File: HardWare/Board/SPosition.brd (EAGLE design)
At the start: 60 x 110 mm, 72 parts

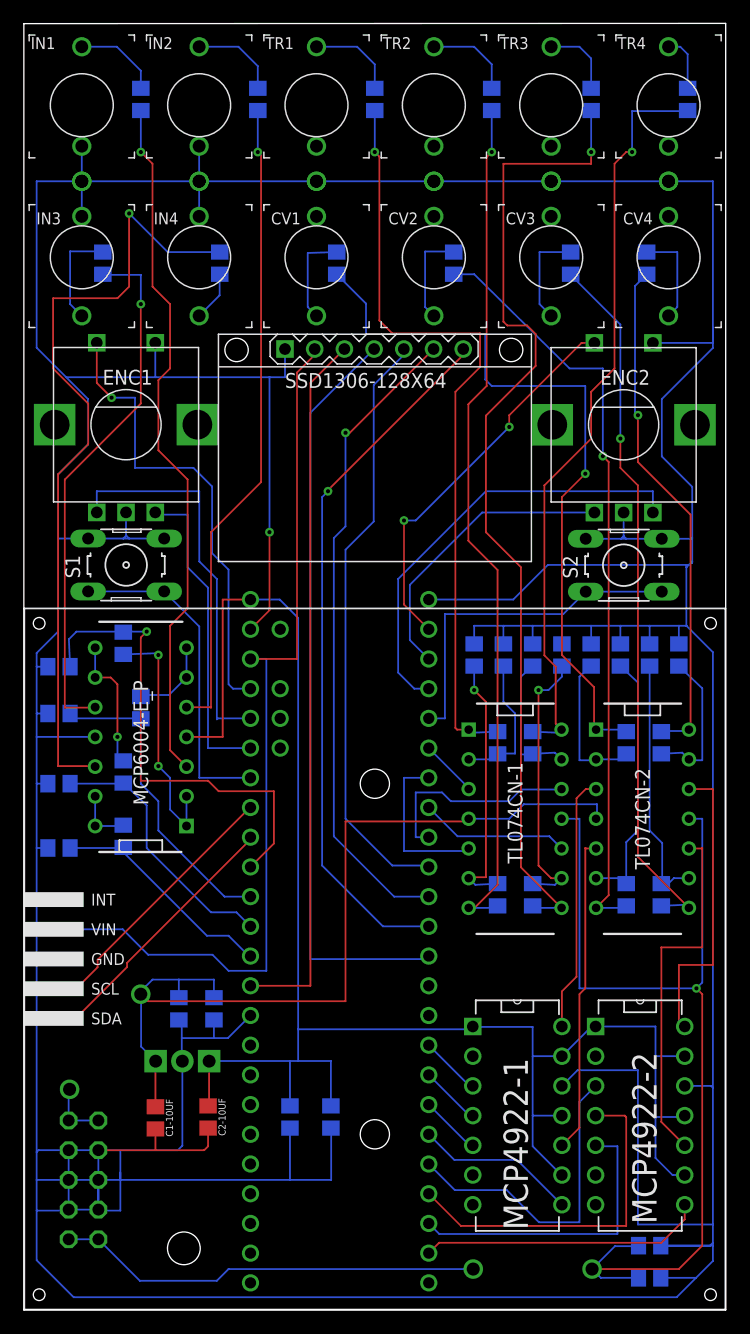
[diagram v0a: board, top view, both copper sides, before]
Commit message: pcb rev5
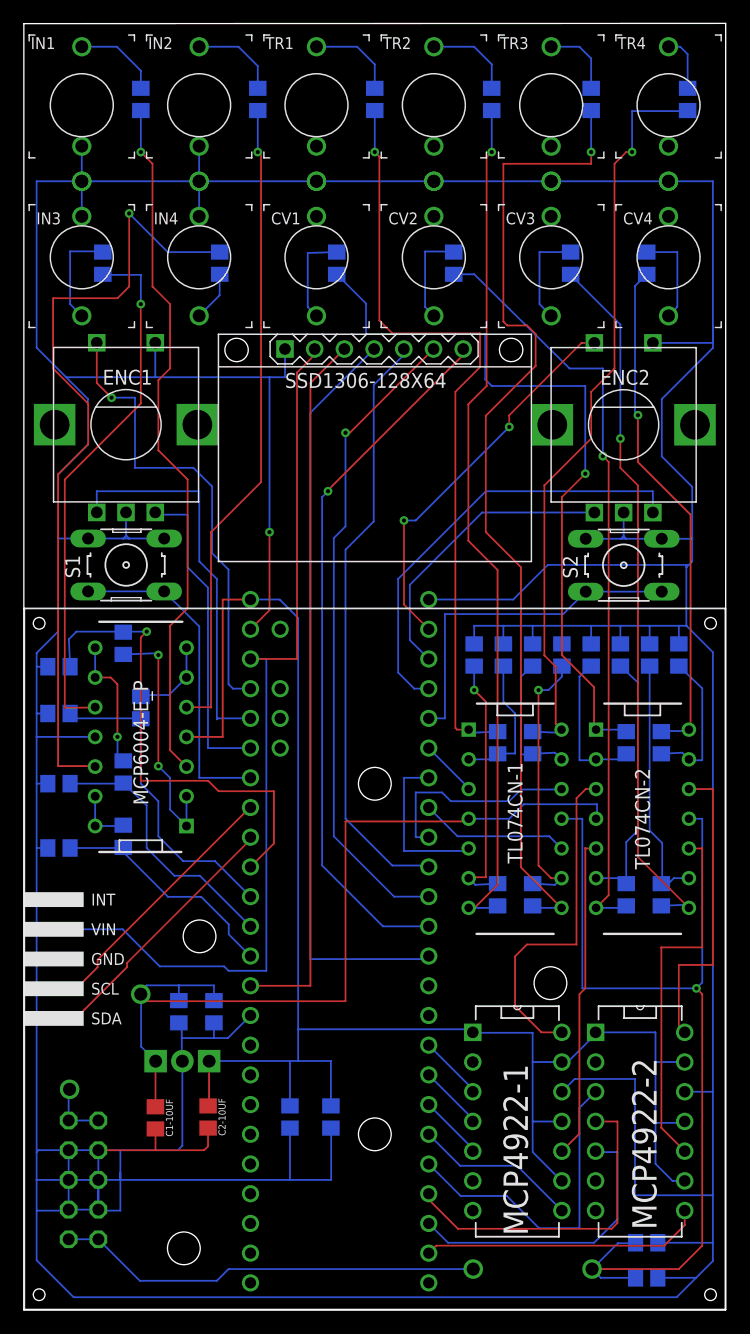
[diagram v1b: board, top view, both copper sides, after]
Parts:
- U$4: value SPREV3 -> SPREV5; device Adafruit Trellis:SPREV3 -> Adafruit Trellis:SPREV5
- moved MCP4922-1 0.50 mm to (46.0, 8.50)
- moved MCP4922-2 0.50 mm to (56.5, 8.50)
- moved C8-100N 0.35 mm to (53.2, 5.75)
- moved C5-100N 0.25 mm to (13.2, 25.5)
- moved C6-100N 0.25 mm to (16.2, 25.5)
- moved C7-100N 0.25 mm to (53.2, 2.75)
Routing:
- net GND: track 611.8 -> 603.7 mm
- net CV1: track 22.0 -> 29.3 mm
- net DAC2SCK: track 30.0 -> 28.4 mm
- net VCC: track 76.8 -> 76.0 mm
- net DAC2MOSI: track 25.9 -> 25.3 mm
- net CV4: track 30.9 -> 31.4 mm
- net CV3: track 25.4 -> 25.9 mm
- net CV2: track 27.2 -> 27.7 mm
